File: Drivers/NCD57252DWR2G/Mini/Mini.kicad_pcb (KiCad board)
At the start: 2 copper layers, 22.8 x 37.6 mm, 18 parts, among them J2 Output, J3 Input, U1 NCD57252DWR2G

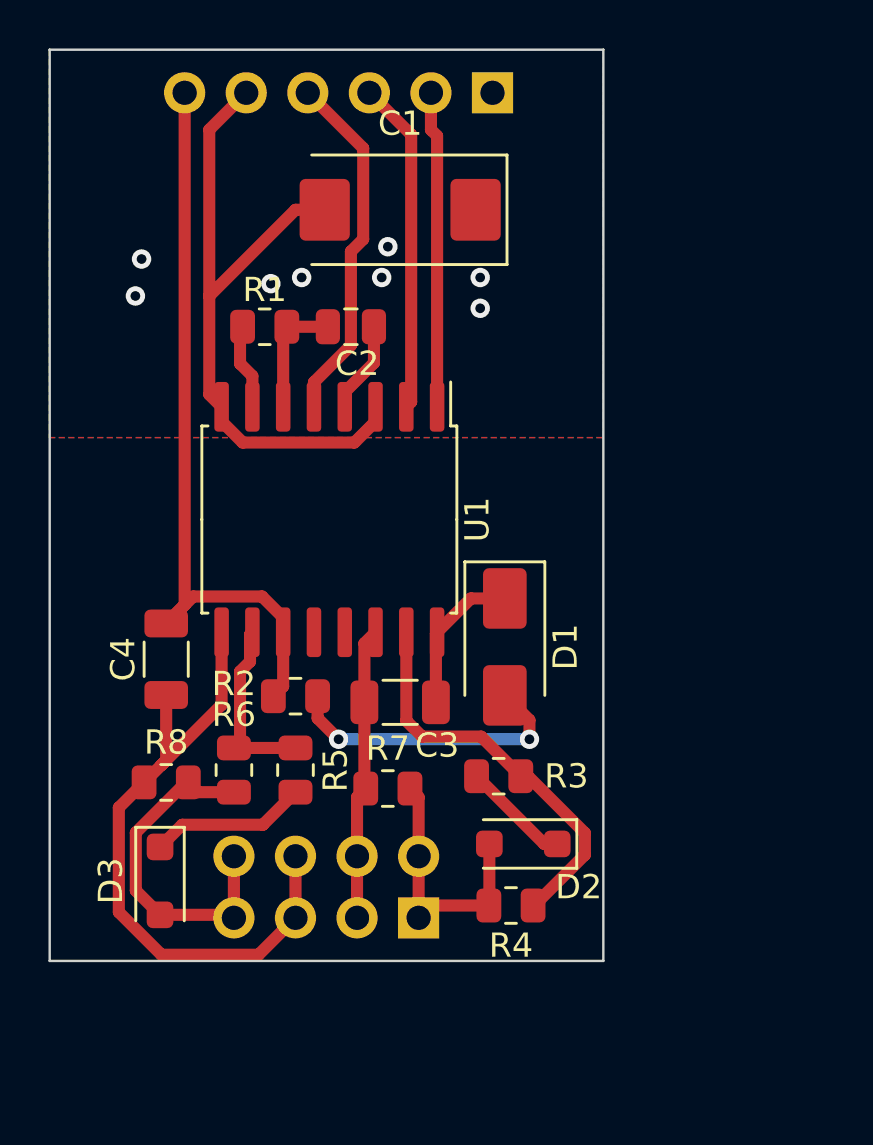
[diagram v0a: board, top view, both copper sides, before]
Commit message: routed_again
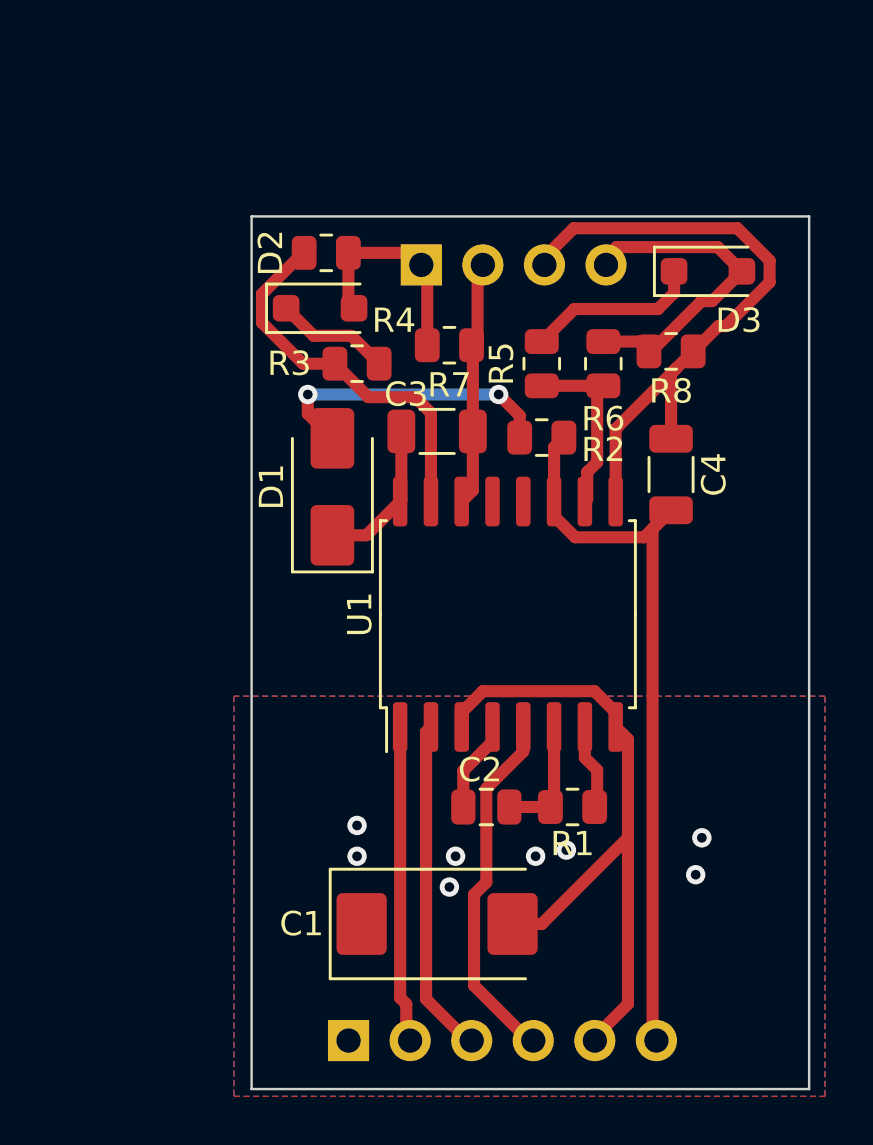
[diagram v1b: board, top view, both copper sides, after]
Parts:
- removed J2: Output, Connector_PinHeader_2.54mm:PinHeader_2x04_P2.54mm_Vertical
- added J1: Output, Connector_PinHeader_2.54mm:PinHeader_1x04_P2.54mm_Vertical, B.Cu at (136.0, 96.0)
- moved J3 39.5 mm to (133.0, 128.0), turned to -90 degrees
- moved D3 33.8 mm to (147.8, 96.3), turned to 0 degrees
- moved C1 29.5 mm to (136.7, 123.2), turned to 0 degrees
- moved R4 28.0 mm to (132.1, 95.5), turned to 0 degrees
- moved R8 27.4 mm to (146.3, 99.6), turned to 180 degrees
- moved D2 23.6 mm to (131.8, 97.8), turned to 0 degrees
- moved R1 23.5 mm to (142.2, 118.4), turned to 0 degrees
- moved R6 22.7 mm to (143.5, 100.1), turned to 90 degrees
- moved C4 22.2 mm to (146.3, 104.6), turned to 90 degrees
- moved C2 20.6 mm to (138.7, 118.4), turned to 180 degrees
- moved R5 19.6 mm to (141.0, 100.1), turned to 90 degrees
- moved R7 18.5 mm to (137.2, 99.3), turned to 180 degrees
- moved R3 18.0 mm to (133.3, 100.1), turned to 0 degrees
- moved R2 14.7 mm to (141.0, 103.1), turned to 180 degrees
- moved C3 11.3 mm to (136.7, 102.9), turned to 0 degrees
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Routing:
- net /PH: track 11.1 -> 8.93 mm
- net /PHASE: track 12.1 -> 10.2 mm
- net /CSR_P: track 27.5 -> 26.4 mm
- net Net-(U1-OutA): track 16.8 -> 15.8 mm
- net /PL: track 14.5 -> 13.8 mm
- net Net-(D3-K): track 6.52 -> 7.18 mm
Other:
- board size 22.8 x 37.6 mm -> 23 x 36 mm
